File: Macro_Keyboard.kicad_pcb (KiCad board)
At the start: 4 copper layers, 95.6 x 84.2 mm, 106 parts, among them J1 USB_C_Receptacle_USB2.0, J2 USB_A, J3 USB_A, J4 USB_A, SW1 SW_Push, SW10 SW_DIP_x01, SW2 SW_DIP_x01, SW3 SW_DIP_x01, SW4 SW_DIP_x01, SW5 SW_DIP_x01, SW6 SW_DIP_x01, SW7 SW_DIP_x01, SW8 SW_DIP_x01, SW9 SW_DIP_x01, U1 STM32L432KCUx, U2 LD39050PU33R, U5 SRV05-4, U6 SRV05-4, Y1 12MHz

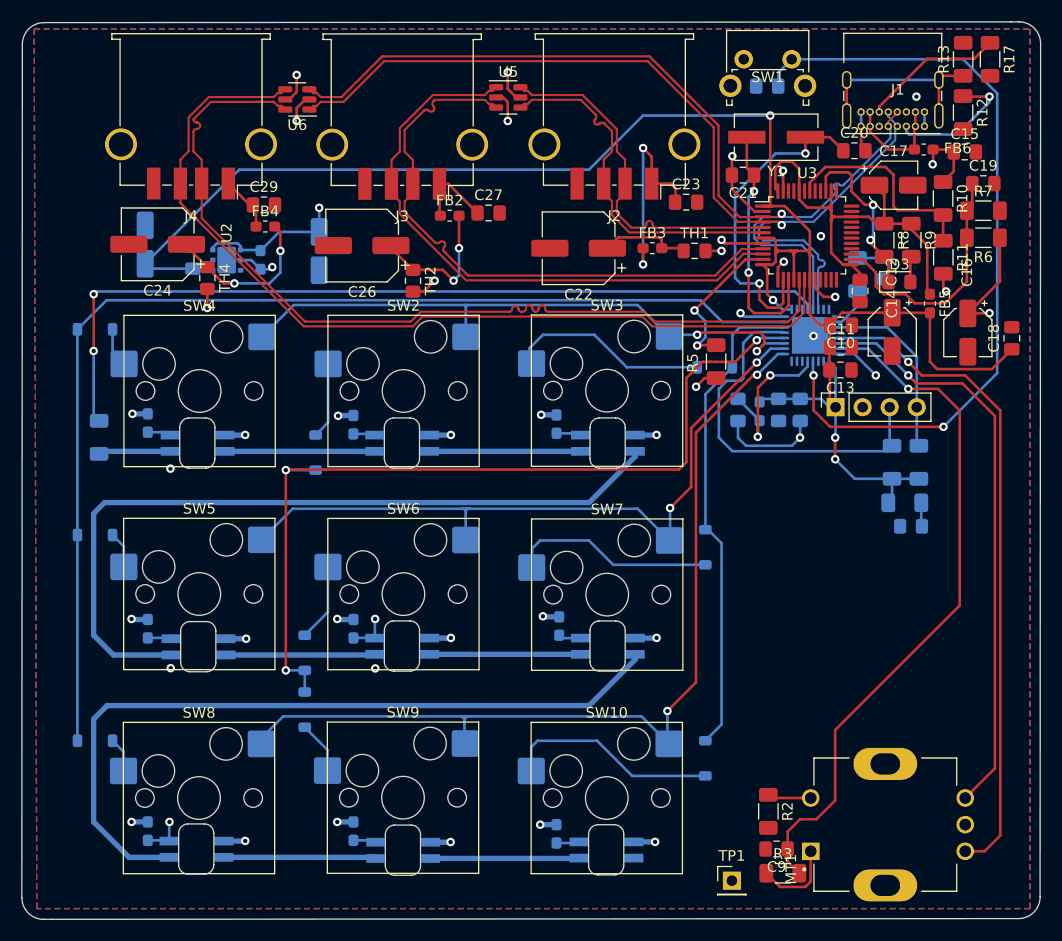
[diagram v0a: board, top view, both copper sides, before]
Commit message: Add files via upload
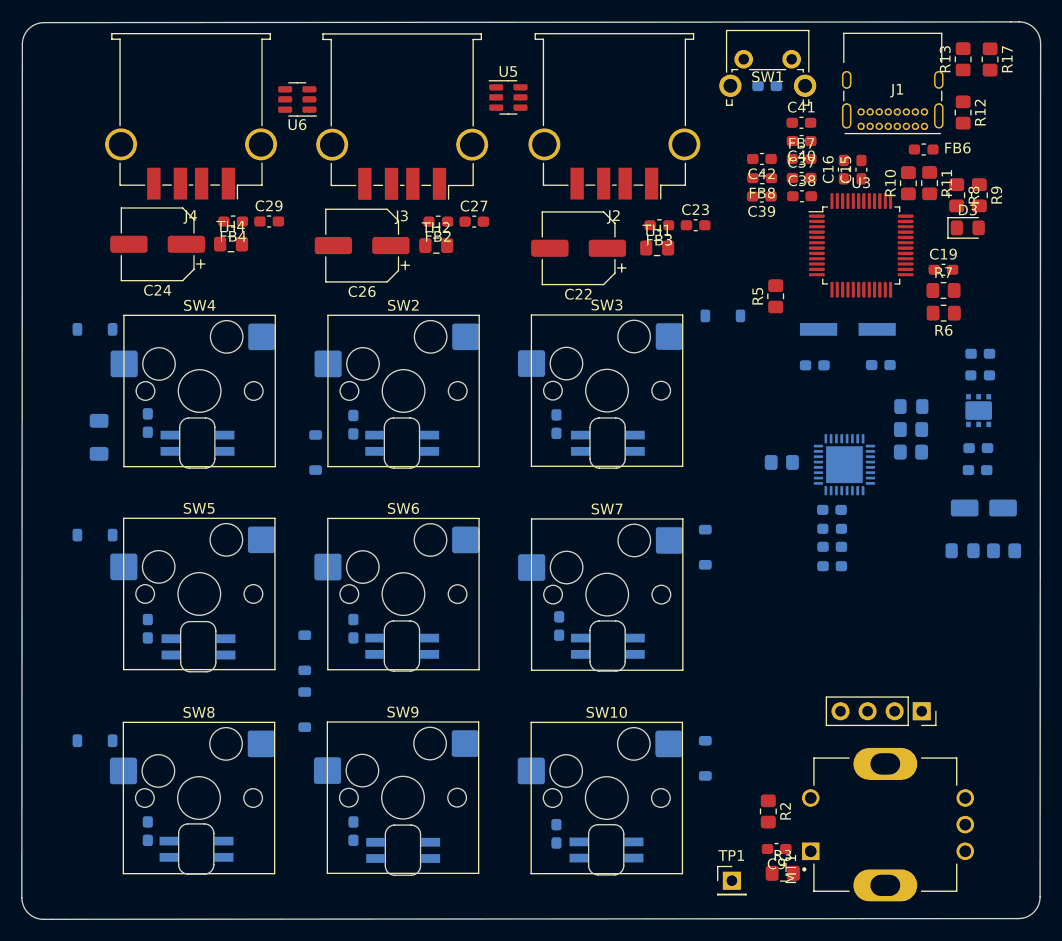
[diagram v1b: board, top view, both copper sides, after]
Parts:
- removed C10, C11, C13, C18: 0.1uF, Capacitor_SMD:C_0805_2012Metric_Pad1.18x1.45mm_HandSolder
- removed C12: 1uF, Capacitor_SMD:CP_Elec_4x5.4
- removed C17: 10uF, Capacitor_SMD:CP_Elec_4x5.8
- removed FB5: BLM18BA, Inductor_SMD:L_0603_1608Metric_Pad1.05x0.95mm_HandSolder
- added C37: 1uF, Capacitor_SMD:C_0603_1608Metric_Pad1.08x0.95mm_HandSolder, F.Cu at (134.5, 54.4)
- added C38: 1uF, Capacitor_SMD:C_0603_1608Metric_Pad1.08x0.95mm_HandSolder, F.Cu at (134.6, 56.1)
- added C39: 1uF, Capacitor_SMD:C_0603_1608Metric_Pad1.08x0.95mm_HandSolder, F.Cu at (130.8, 56.1)
- added C40: 1uF, Capacitor_SMD:C_0603_1608Metric_Pad1.08x0.95mm_HandSolder, F.Cu at (134.5, 50.9)
- added C41: 0.1uF, Capacitor_SMD:C_0603_1608Metric_Pad1.08x0.95mm_HandSolder, F.Cu at (134.5, 49.2)
- added C42: 0.1uF, Capacitor_SMD:C_0603_1608Metric_Pad1.08x0.95mm_HandSolder, F.Cu at (130.8, 52.6)
- added FB7: BLM18BA, Inductor_SMD:L_0603_1608Metric_Pad1.05x0.95mm_HandSolder, F.Cu at (134.5, 52.6)
- added FB8: BLM18BA, Inductor_SMD:L_0603_1608Metric_Pad1.05x0.95mm_HandSolder, F.Cu at (130.8, 54.4)
- C14: value 0.1uF -> 10uF; footprint Capacitor_SMD:C_0805_2012Metric_Pad1.18x1.45mm_HandSolder -> Capacitor_SMD:CP_Elec_4x5.8; moved to B.Cu
- C15, C19, C23, C27, C29, C4, C5, C6, C7, C8, C9: footprint Capacitor_SMD:C_0805_2012Metric_Pad1.18x1.45mm_HandSolder -> Capacitor_SMD:C_0603_1608Metric_Pad1.08x0.95mm_HandSolder
- C16, C2, C3: footprint Capacitor_SMD:CP_Elec_4x5.4 -> Capacitor_SMD:C_0603_1608Metric_Pad1.08x0.95mm_HandSolder
- C20, C21: footprint Capacitor_SMD:C_0805_2012Metric_Pad1.18x1.45mm_HandSolder -> Capacitor_SMD:C_0603_1608Metric_Pad1.08x0.95mm_HandSolder; moved to B.Cu
- R1, R10, R11, R12, R13, R15, R16, R17, R2, R3, R4, R5, R6, R7, R8, R9: footprint Resistor_SMD:R_1206_3216Metric_Pad1.30x1.75mm_HandSolder -> Resistor_SMD:R_0805_2012Metric_Pad1.20x1.40mm_HandSolder
- Y1: moved to B.Cu
- moved C3 80.9 mm to (151.0, 81.8), turned to 180 degrees
- moved C4 75.9 mm to (151.1, 79.7), turned to 180 degrees
- moved U2 72.0 mm to (151.1, 76.2), turned to 0 degrees
- moved C1 68.4 mm to (151.3, 72.9), turned to 0 degrees
- moved C2 62.8 mm to (151.3, 70.9), turned to 0 degrees
- moved U4 29.7 mm to (145.8, 104.4), turned to -90 degrees
- moved C14 23.4 mm to (151.6, 85.3), turned to 180 degrees
- moved C21 22.0 mm to (142.0, 71.9), turned to 0 degrees
- moved C20 20.5 mm to (135.7, 72.0), turned to 180 degrees
- moved Y1 19.2 mm to (138.9, 68.6), turned to 0 degrees
- moved C16 19.2 mm to (138.5, 53.6), turned to 90 degrees
- moved R4 15.4 mm to (144.8, 78.0), turned to 0 degrees
- moved C6 15.0 mm to (137.4, 90.8), turned to 180 degrees
- moved C7 13.8 mm to (137.4, 89.0), turned to 180 degrees
- moved D2 13.2 mm to (144.8, 75.8), turned to 0 degrees
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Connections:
- C14 pad 1: DVDD -> +3.3V
- U3 pad 1: +3.3V -> AVDD
- U3 pad 12: +3.3V -> AVDD
- U3 pad 16: +3.3V -> AVDD
- U3 pad 19: +3.3V -> AVDD
- U3 pad 7: +3.3V -> AVDD
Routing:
- net +3.3V: track 174.9 -> 0.00 mm, vias 4 -> 0
- net COL 0: track 106.9 -> 0.00 mm
- net USBD_N: track 88.9 -> 0.00 mm, vias 1 -> 0
- net USBD_P: track 88.9 -> 0.00 mm, vias 1 -> 0
- net /USB/D_P3: track 86.2 -> 0.00 mm
- net /USB/D_N3: track 86.0 -> 0.00 mm
- net ROW 2: track 85.7 -> 0.00 mm, vias 2 -> 0
- net COL 1: track 81.9 -> 0.00 mm, vias 3 -> 0
- net LED: track 80.2 -> 0.00 mm, vias 2 -> 0
- net +5V: track 75.9 -> 0.00 mm, vias 27 -> 0
- net GND: track 75.5 -> 0.00 mm, vias 20 -> 0
- net Net-(U1-NRST): track 74.5 -> 0.00 mm, vias 2 -> 0
- net Net-(SK6812MINI_E3-DOUT): track 73.0 -> 0.00 mm
- net Net-(SK6812MINI_E6-DOUT): track 71.7 -> 0.00 mm
- net ROW 1: track 68.3 -> 0.00 mm, vias 2 -> 0
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- removed copper zone on In2.Cu, net +5V
- removed copper zone on B.Cu, net GND
- removed copper zone on F.Cu, net GND
- removed copper zone on In1.Cu, net GND
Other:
- board text removed: "TODO if Route is okay: .) Name .) Silkscreen .) DRC"
